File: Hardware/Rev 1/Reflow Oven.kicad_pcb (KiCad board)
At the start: 4 copper layers, 100 x 50 mm, 85 parts, among them IC1 MCP1792T, J1 SW, J10 2350513-2, J11 USB4110-GF-A_REVB, J12 POW_SEL, J13 Conn_01x02, J2 ENC, J3 Adafruit 4101, J4 Adafruit 4101, J5 Adafruit 4101, J6 GC9A01 1.28" TFT, J7 2350513-3, J8 2350513-2, J9 2350513-2, Q1 IRLML2060, Q2 IRLML2060, Q3 IRLML2060, SW1 DNF, SW2 DNF, U1 USBUF02W6, U2 W25Q16JV, U3 FT24C04A, U4 RP2040, Y1 12MHz

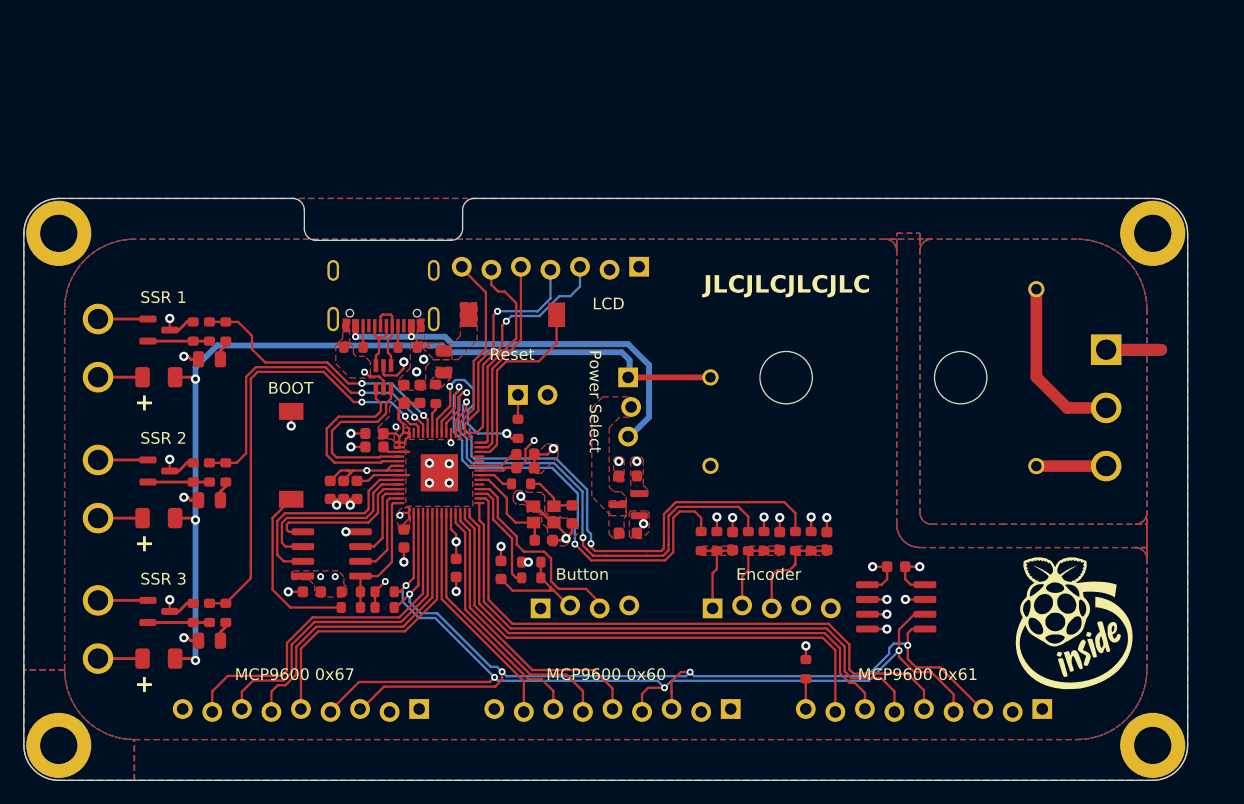
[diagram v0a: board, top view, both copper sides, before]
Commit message: redid 2 layer, thanks git
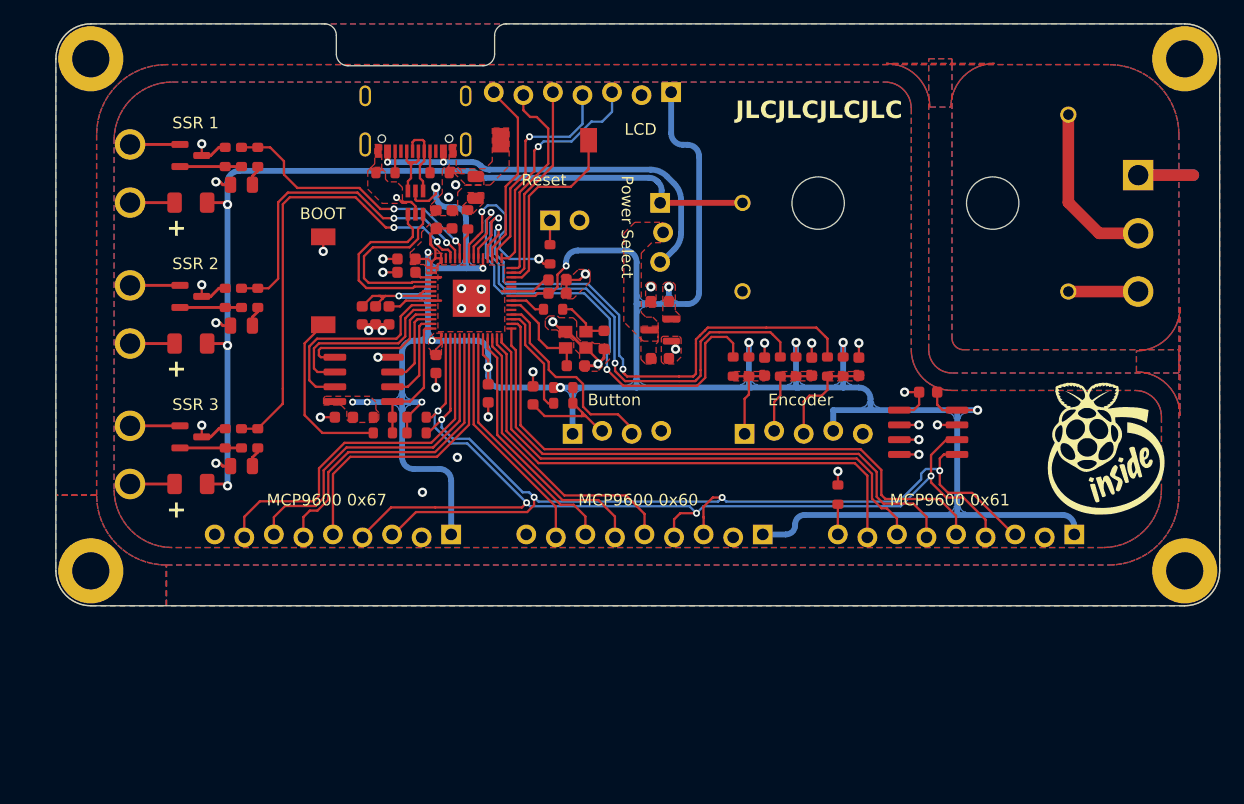
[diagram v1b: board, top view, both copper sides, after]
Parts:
- moved J11 15.3 mm to (131.2, 57.3)
- moved C1 15.2 mm to (161.2, 79.5)
- moved C10 15.2 mm to (143.3, 73.2)
- moved C11 15.2 mm to (125.0, 83.8)
- moved C12 15.2 mm to (137.4, 81.8)
- moved C13 15.2 mm to (134.3, 66.8)
- moved C14 15.2 mm to (132.9, 66.8)
- moved C15 15.2 mm to (152.2, 78.8)
- moved C16 15.2 mm to (127.7, 75.0)
- moved C17 15.2 mm to (126.6, 75.0)
- moved C18 15.2 mm to (132.9, 79.2)
- moved C19 15.2 mm to (130.4, 70.2)
- moved C2 15.2 mm to (165.2, 79.5)
- moved C20 15.2 mm to (175.2, 81.6)
- moved C21 15.2 mm to (152.2, 73.8)
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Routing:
- net +3V3: track 45.3 -> 252.0 mm
- net GND: vias 37 -> 39
- added copper zone on B.Cu, net +3V3
- added copper zone on B.Cu, net GND
- removed copper zone on In1.Cu, net +3V3
- removed copper zone on In2.Cu, net GND
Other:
- copper layers 4 -> 2
